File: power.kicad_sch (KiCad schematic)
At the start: 12 parts, among them U3 L7805, U4 XC6206P332MR

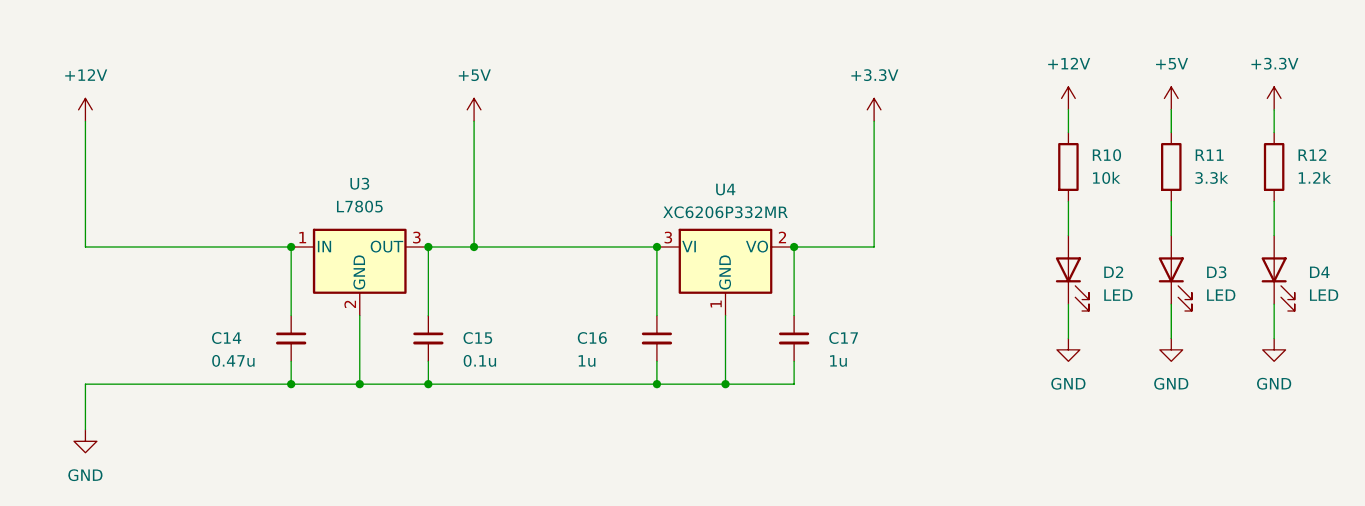
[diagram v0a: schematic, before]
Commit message: v0.2
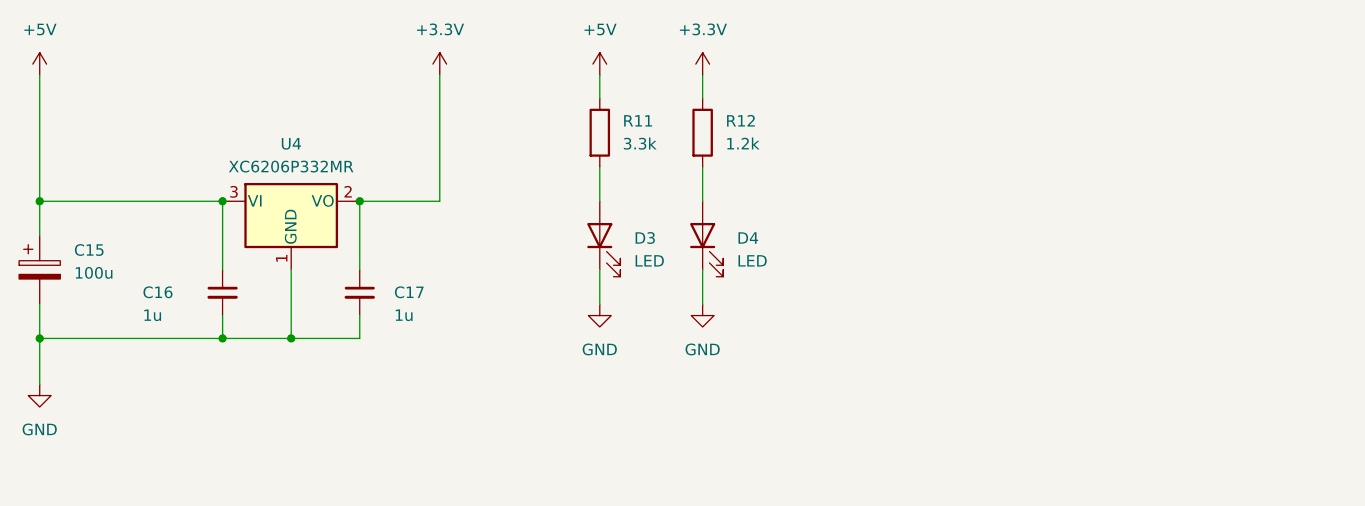
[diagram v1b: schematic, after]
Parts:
- removed C14: 0.47u, Capacitor_SMD:C_0603_1608Metric, symbol Device:C_Small
- removed C15: 0.1u, Capacitor_SMD:C_0603_1608Metric, symbol Device:C_Small
- removed D2: LED, LED_SMD:LED_0603_1608Metric, symbol Device:LED
- removed R10: 10k, Resistor_SMD:R_0603_1608Metric, symbol Device:R
- removed U3: L7805, Package_TO_SOT_SMD:TO-252-2, symbol Regulator_Linear:L7805
- added C15: 100u, Capacitor_THT:C_Radial_D6.3mm_H11.0mm_P2.50mm, symbol Device:C_Polarized
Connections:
- net +5V: now also C15.1
- net GND: now also C15.2
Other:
- moved on the sheet: C16, C17, D3, D4, R11, R12, U4
